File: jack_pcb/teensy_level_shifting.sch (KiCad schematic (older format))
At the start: 6 parts, among them J35 USB_B, U10 Teensy4.1, U6 74125, U7 74125, U8 74125, U9 74125

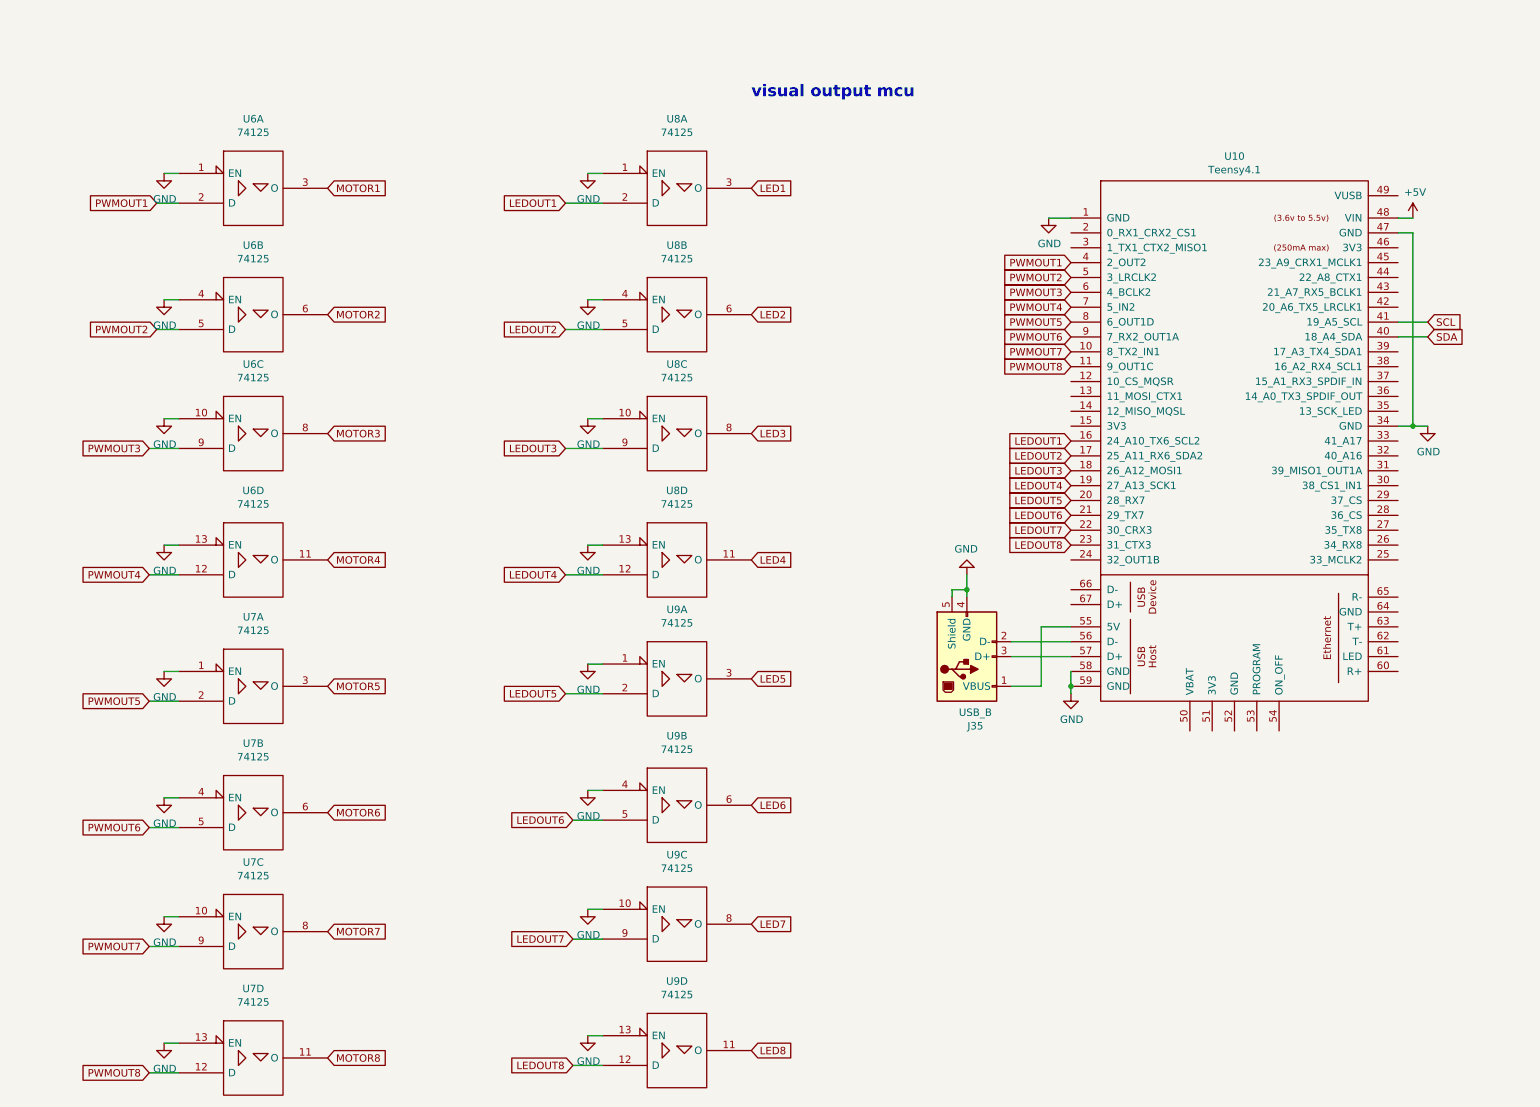
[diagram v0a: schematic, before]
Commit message: finalized jack board
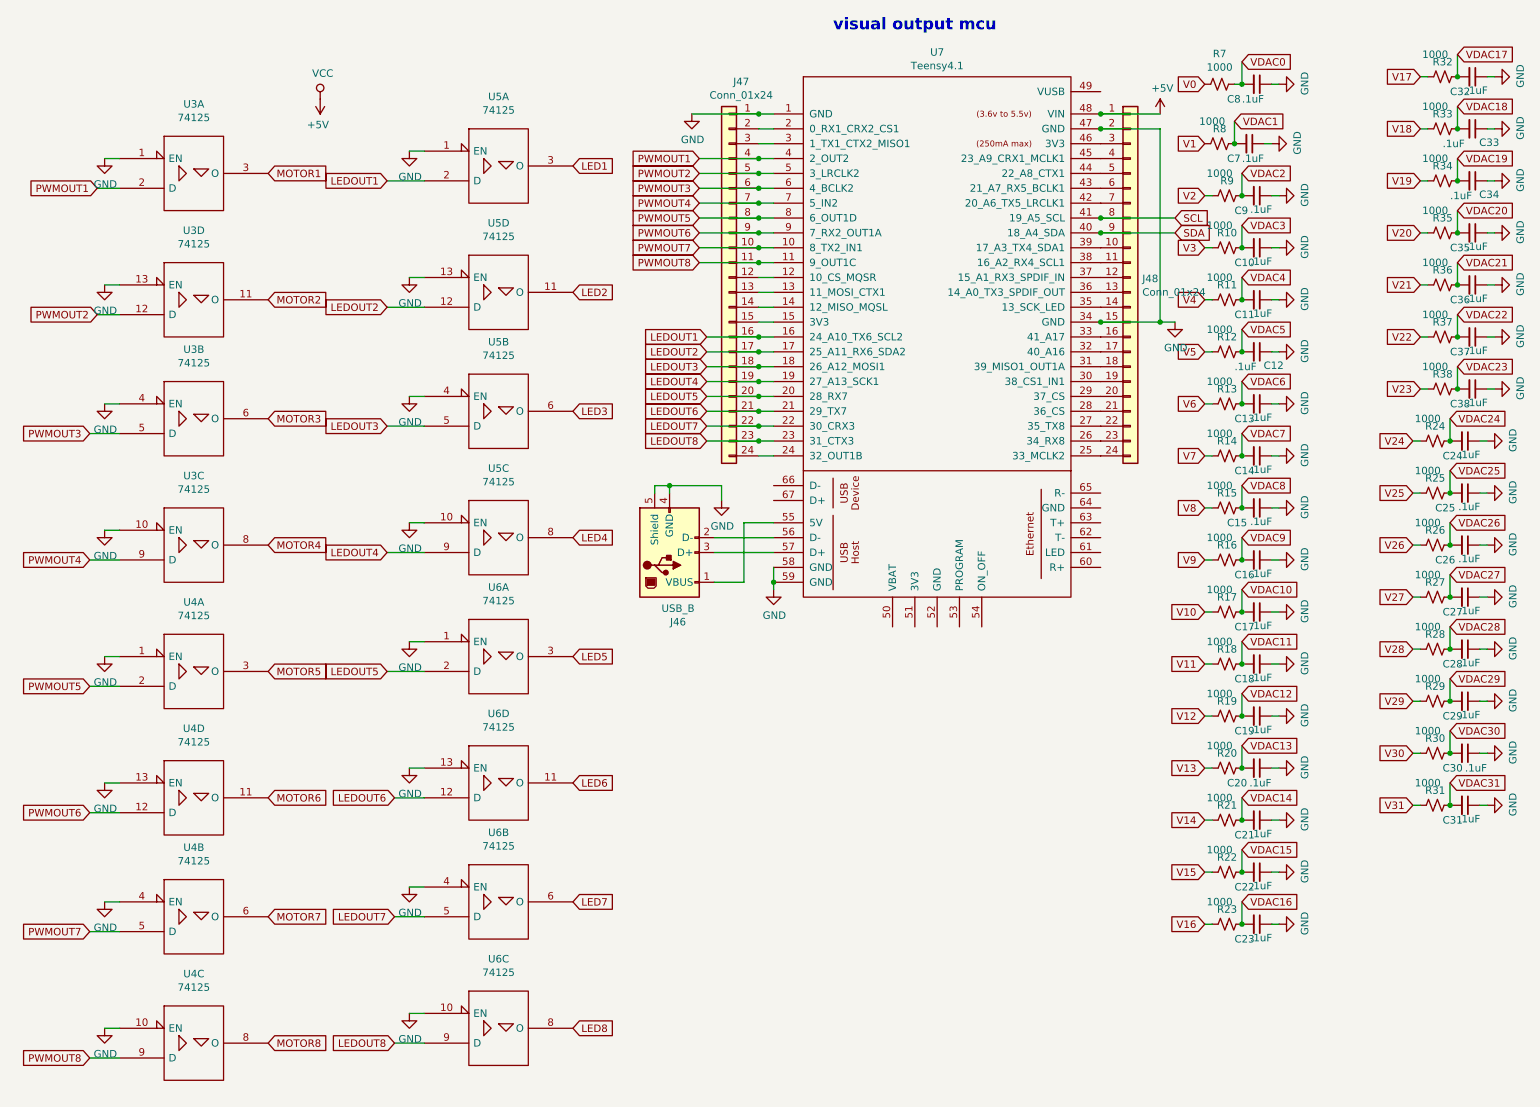
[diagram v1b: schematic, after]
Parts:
- added C10, C11, C12, C13, C14, C15, C16, C17, C18, C19, C20, C21, C22, C23, C24, C25, C26, C27, C28, C29, C30, C31, C32, C33, C34, C35, C36, C37, C38, C7, C8, C9: .1uF, Capacitor_THT:C_Axial_L3.8mm_D2.6mm_P7.50mm_Horizontal, symbol Device:C_Small
- added J47, J48: Conn_01x24, Connector_PinHeader_2.54mm:PinHeader_1x24_P2.54mm_Vertical, symbol Connector_Generic:Conn_01x24
- added R10, R11, R12, R13, R14, R15, R16, R17, R18, R19, R20, R21, R22, R23, R24, R25, R26, R27, R28, R29, R30, R31, R32, R33, R34, R35, R36, R37, R38, R7, R8, R9: 1000, Resistor_THT:R_Axial_DIN0207_L6.3mm_D2.5mm_P10.16mm_Horizontal, symbol Device:R_Small_US
- renumbered J35 to J46, U6 to U3, U7 to U4, U8 to U5, U9 to U6, U10 to U7
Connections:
- net VCC is gone; now on net +5V: U3.14 (VCC), U3.14 (VCC), U3.14 (VCC), U3.14 (VCC), U4.14 (VCC), U4.14 (VCC), U4.14 (VCC), U4.14 (VCC), U5.14 (VCC), U5.14 (VCC), U5.14 (VCC), U5.14 (VCC), U6.14 (VCC), U6.14 (VCC), U6.14 (VCC), U6.14 (VCC)
- net +5V: now also J48.1 (Pin_1)
- net GND: now also C10.1, C11.1, C12.1, C13.1, C14.1, C15.1, C16.1, C17.1, C18.1, C19.1, C20.1, C21.1, C22.1, C23.1, C24.1, C25.1, C26.1, C27.1, C28.1, C29.1, C30.1, C31.1, C32.1, C33.1, C34.1, C35.1, C36.1, C37.1, C38.1, C7.1, C8.1, C9.1, J47.1 (Pin_1), J48.15 (Pin_15), J48.2 (Pin_2)
- net LED2: now also U5.11 (O); no longer U5.6 (O)
- net LED3: now also U5.6 (O); no longer U5.8 (O)
- net LED4: now also U5.8 (O); no longer U5.11 (O)
- net LED6: now also U6.11 (O); no longer U6.6 (O)
- net LED7: now also U6.6 (O); no longer U6.8 (O)
- net LED8: now also U6.8 (O); no longer U6.11 (O)
- net LEDOUT1: now also J47.16 (Pin_16)
- net LEDOUT2: now also U5.12 (D), J47.17 (Pin_17); no longer U5.5 (D)
- net LEDOUT3: now also U5.5 (D), J47.18 (Pin_18); no longer U5.9 (D)
- net LEDOUT4: now also U5.9 (D), J47.19 (Pin_19); no longer U5.12 (D)
- net LEDOUT5: now also J47.20 (Pin_20)
- net LEDOUT6: now also U6.12 (D), J47.21 (Pin_21); no longer U6.5 (D)
- net LEDOUT7: now also U6.5 (D), J47.22 (Pin_22); no longer U6.9 (D)
- net LEDOUT8: now also U6.9 (D), J47.23 (Pin_23); no longer U6.12 (D)
- net MOTOR2: now also U3.11 (O); no longer U3.6 (O)
- net MOTOR3: now also U3.6 (O); no longer U3.8 (O)
- net MOTOR4: now also U3.8 (O); no longer U3.11 (O)
- net MOTOR6: now also U4.11 (O); no longer U4.6 (O)
- net MOTOR7: now also U4.6 (O); no longer U4.8 (O)
- net MOTOR8: now also U4.8 (O); no longer U4.11 (O)
- net PWMOUT1: now also J47.4 (Pin_4)
- net PWMOUT2: now also U3.12 (D), J47.5 (Pin_5); no longer U3.5 (D)
- net PWMOUT3: now also U3.5 (D), J47.6 (Pin_6); no longer U3.9 (D)
- net PWMOUT4: now also U3.9 (D), J47.7 (Pin_7); no longer U3.12 (D)
- net PWMOUT5: now also J47.8 (Pin_8)
- net PWMOUT6: now also U4.12 (D), J47.9 (Pin_9); no longer U4.5 (D)
- net PWMOUT7: now also U4.5 (D), J47.10 (Pin_10); no longer U4.9 (D)
- net PWMOUT8: now also U4.9 (D), J47.11 (Pin_11); no longer U4.12 (D)
- net SCL: now also J48.8 (Pin_8)
- net SDA: now also J48.9 (Pin_9)
- net at U7.12 (10_CS_MQSR): now also J47.12 (Pin_12)
- net at U7.13 (11_MOSI_CTX1): now also J47.13 (Pin_13)
- net at U7.14 (12_MISO_MQSL): now also J47.14 (Pin_14)
- net at U7.15 (3V3): now also J47.15 (Pin_15)
- net at U7.2 (0_RX1_CRX2_CS1): now also J47.2 (Pin_2)
- net at U7.24 (32_OUT1B): now also J47.24 (Pin_24)
- net at U7.25 (33_MCLK2): now also J48.24 (Pin_24)
- net at U7.26 (34_RX8): now also J48.23 (Pin_23)
- net at U7.27 (35_TX8): now also J48.22 (Pin_22)
- net at U7.28 (36_CS): now also J48.21 (Pin_21)
- net at U7.29 (37_CS): now also J48.20 (Pin_20)
- net at U7.3 (1_TX1_CTX2_MISO1): now also J47.3 (Pin_3)
- net at U7.30 (38_CS1_IN1): now also J48.19 (Pin_19)
- net at U7.31 (39_MISO1_OUT1A): now also J48.18 (Pin_18)
- net at U7.32 (40_A16): now also J48.17 (Pin_17)
- net at U7.33 (41_A17): now also J48.16 (Pin_16)
- net at U7.35 (13_SCK_LED): now also J48.14 (Pin_14)
- net at U7.36 (14_A0_TX3_SPDIF_OUT): now also J48.13 (Pin_13)
- net at U7.37 (15_A1_RX3_SPDIF_IN): now also J48.12 (Pin_12)
- net at U7.38 (16_A2_RX4_SCL1): now also J48.11 (Pin_11)
- net at U7.39 (17_A3_TX4_SDA1): now also J48.10 (Pin_10)
- net at U7.42 (20_A6_TX5_LRCLK1): now also J48.7 (Pin_7)
- net at U7.43 (21_A7_RX5_BCLK1): now also J48.6 (Pin_6)
- net at U7.44 (22_A8_CTX1): now also J48.5 (Pin_5)
- net at U7.45 (23_A9_CRX1_MCLK1): now also J48.4 (Pin_4)
- net at U7.46 (3V3): now also J48.3 (Pin_3)
- new net V0: R7.2
- new net V1: R8.1
- new net V10: R17.1
- new net V11: R18.1
- new net V12: R19.1
- new net V13: R20.1
- new net V14: R21.1
- new net V15: R22.1
- new net V16: R23.1
- new net V17: R32.1
- new net V18: R33.1
- new net V19: R34.1
- new net V2: R9.1
- new net V20: R35.1
- new net V21: R36.1
- new net V22: R37.1
- new net V23: R38.1
- new net V24: R24.1
- new net V25: R25.1
- new net V26: R26.1
- new net V27: R27.1
- new net V28: R28.1
- new net V29: R29.1
- new net V3: R10.1
- new net V30: R30.1
- new net V31: R31.1
- new net V4: R11.1
- new net V5: R12.1
- new net V6: R13.1
- new net V7: R14.1
- new net V8: R15.1
- new net V9: R16.1
- new net VDAC0: C8.2, R7.1
- new net VDAC1: C7.2, R8.2
- new net VDAC10: C17.2, R17.2
- new net VDAC11: C18.2, R18.2
- new net VDAC12: C19.2, R19.2
- new net VDAC13: C20.2, R20.2
- new net VDAC14: C21.2, R21.2
- new net VDAC15: C22.2, R22.2
- new net VDAC16: C23.2, R23.2
- new net VDAC17: C32.2, R32.2
- new net VDAC18: C33.2, R33.2
- new net VDAC19: C34.2, R34.2
- new net VDAC2: C9.2, R9.2
- new net VDAC20: C35.2, R35.2
- new net VDAC21: C36.2, R36.2
- new net VDAC22: C37.2, R37.2
- new net VDAC23: C38.2, R38.2
- new net VDAC24: C24.2, R24.2
- new net VDAC25: C25.2, R25.2
- new net VDAC26: C26.2, R26.2
- new net VDAC27: C27.2, R27.2
- new net VDAC28: C28.2, R28.2
- new net VDAC29: C29.2, R29.2
- new net VDAC3: C10.2, R10.2
- new net VDAC30: C30.2, R30.2
- new net VDAC31: C31.2, R31.2
- new net VDAC4: C11.2, R11.2
- new net VDAC5: C12.2, R12.2
- new net VDAC6: C13.2, R13.2
- new net VDAC7: C14.2, R14.2
- new net VDAC8: C15.2, R15.2
- new net VDAC9: C16.2, R16.2
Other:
- moved on the sheet: J46, U3A, U3B, U3C, U3D, U4A, U4B, U4C, U4D, U5A, U5B, U5C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
